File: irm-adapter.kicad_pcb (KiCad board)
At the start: 2 copper layers, 80 x 40 mm, 9 parts, among them J1 L, J2 Vout, J3 N, J4 Conn_01x04_Male, J5 Conn_01x04_Male, J6 Conn_01x04_Female, J7 Conn_01x04_Female

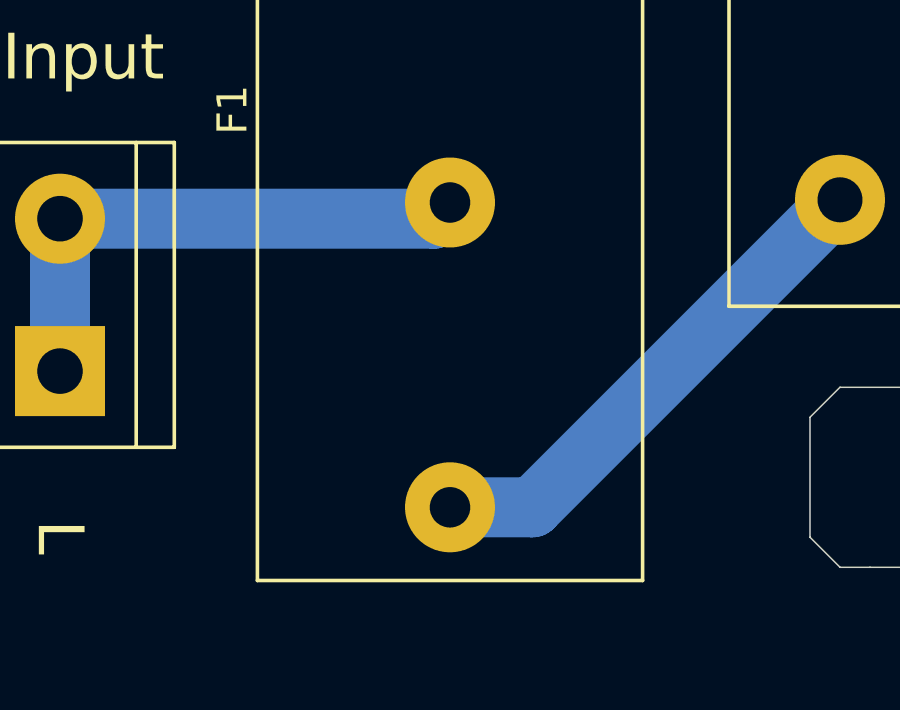
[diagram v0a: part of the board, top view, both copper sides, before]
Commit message: changes
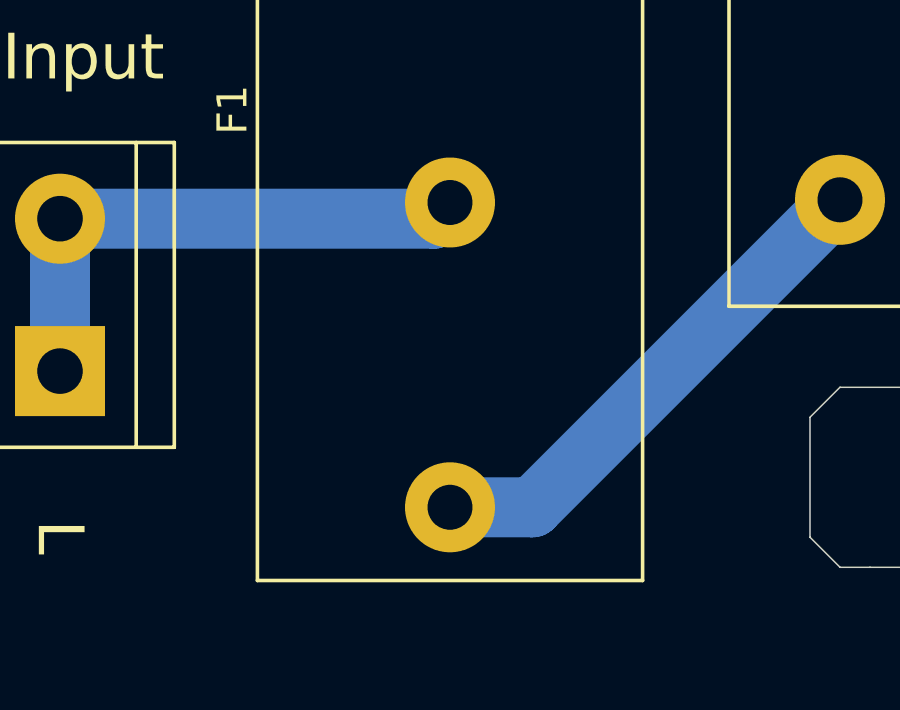
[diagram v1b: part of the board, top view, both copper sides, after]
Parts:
- J4, J5: value Conn_01x04_Male -> 1x4
- J6, J7: value Conn_01x04_Female -> 1x4
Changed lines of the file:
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@@
-(kicad_pcb (version 20171130) (host pcbnew "(5.1.0)-1")
+(kicad_pcb (version 20171130) (host pcbnew 5.1.2)
   (general
     (thickness 1.6)
@@
     (mod_text_size 1 1)
     (mod_text_width 0.15)
-    (pad_size 1.524 1.524)
-    (pad_drill 0.762)
+    (pad_size 3 3)
+    (pad_drill 1.5)
     (pad_to_mask_clearance 0.051)
     (solder_mask_min_width 0.25)
@@
     (fp_line (start 32.9 6.42) (end 32.9 -6.42) (layer F.SilkS) (width 0.12))
     (fp_line (start 32.9 6.42) (end -2.44 6.42) (layer F.SilkS) (width 0.12))
-    (pad 2 thru_hole circle (at 10.16 0 90) (size 3 3) (drill 1.35) (layers *.Cu *.Mask)
+    (pad 2 thru_hole circle (at 10.16 0 90) (size 3 3) (drill 1.5) (layers *.Cu *.Mask)
       (net 1 /L))
-    (pad 1 thru_hole circle (at 0 0 90) (size 3 3) (drill 1.35) (layers *.Cu *.Mask)
+    (pad 1 thru_hole circle (at 0 0 90) (size 3 3) (drill 1.5) (layers *.Cu *.Mask)
       (net 5 /L_F))
     (model ${KISYS3DMOD}/Fuse.3dshapes/Fuseholder_Cylinder-5x20mm_Bulgin_FX0457_Horizontal_Closed.wrl
@@
       (effects (font (size 1 1) (thickness 0.15)))
     )
-    (fp_text value Conn_01x04_Male (at 0 9.95 180) (layer F.Fab)
+    (fp_text value 1x4 (at 0 9.95 180) (layer F.Fab)
       (effects (font (size 1 1) (thickness 0.15)))
     )
@@
       (effects (font (size 1 1) (thickness 0.15)))
     )
-    (fp_text value Conn_01x04_Male (at 0 9.95 180) (layer F.Fab)
+    (fp_text value 1x4 (at 0 9.95 180) (layer F.Fab)
       (effects (font (size 1 1) (thickness 0.15)))
     )
@@
       (effects (font (size 1 1) (thickness 0.15)))
     )
-    (fp_text value Conn_01x04_Female (at 0 10.39 180) (layer F.Fab)
+    (fp_text value 1x4 (at 0 10.39 180) (layer F.Fab)
       (effects (font (size 1 1) (thickness 0.15)))
     )
@@
       (effects (font (size 1 1) (thickness 0.15)))
     )
-    (fp_text value Conn_01x04_Female (at 0 10.39 180) (layer F.Fab)
-      (effects (font (size 1 1) (thickness 0.15)))
-    )
+    (fp_text value 1x4 (at 0 10.39 180) (layer F.Fab)
+      (effects (font (size 1 1) (thickness 0.15)))
+    )
